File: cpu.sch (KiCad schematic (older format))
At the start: 6 parts

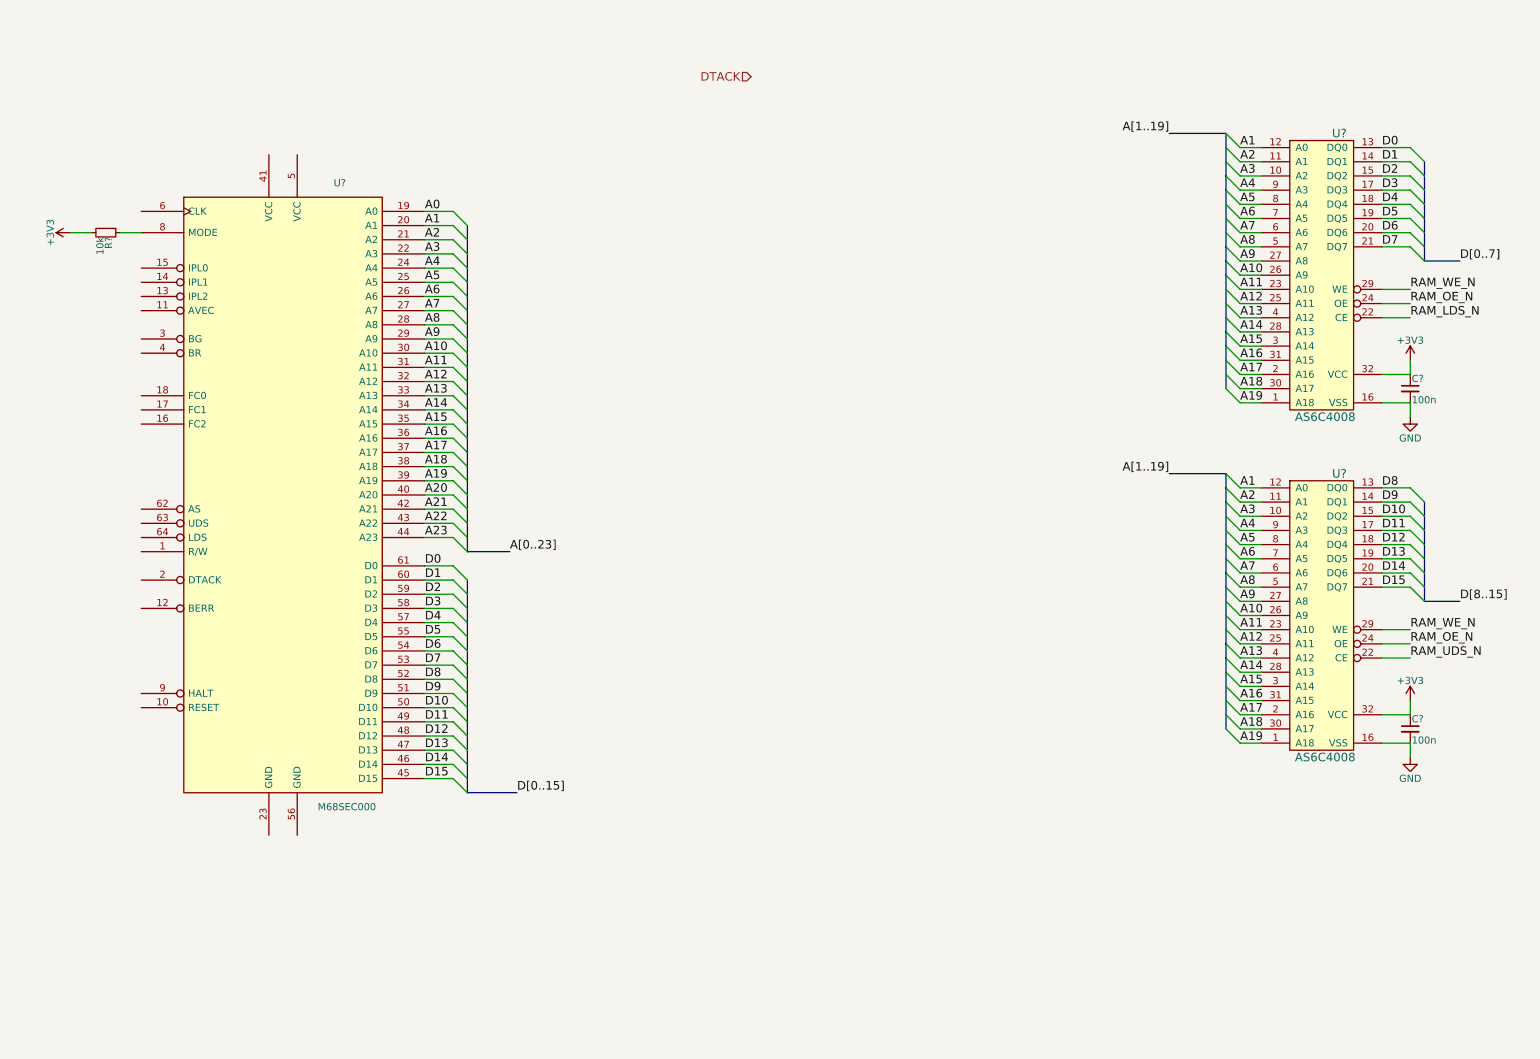
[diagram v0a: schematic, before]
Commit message: boot process
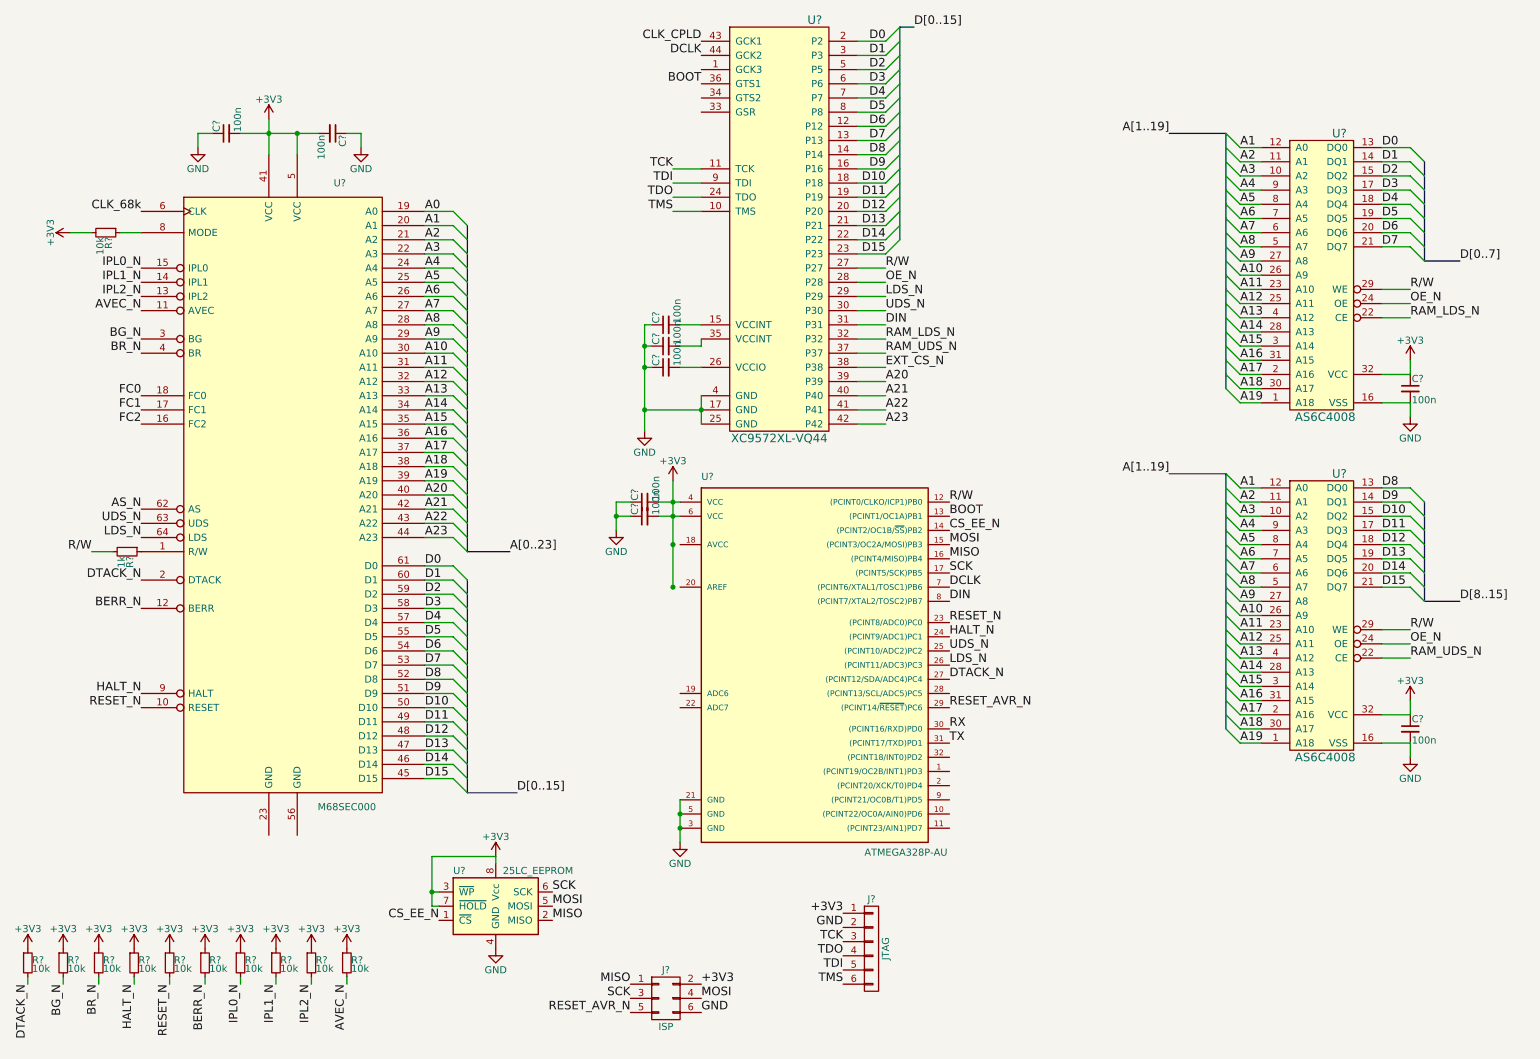
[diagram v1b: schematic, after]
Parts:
- added C? (x7): 100n, symbol C_Small
- added J?: JTAG, symbol CONN_01X06
- added J?: ISP, symbol CONN_02X03
- added R?: 1k, symbol R_Small
- added R? (x10): 10k, symbol R_Small
- added U?: XC9572XL-VQ44, symbol XC9572XL-VQ44
- added U?: ATMEGA328P-AU, TQFP32, symbol ATMEGA328P-AU
- added U?: 25LC_EEPROM, symbol 25LC_EEPROM
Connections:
- net +3V3: now also U?.41 (VCC), U?.5 (VCC), C?.2, C?.2, C?.2, C?.2, J?.1 (P1), J?.2 (P2), R?.1, R?.1, R?.1, R?.1, R?.1, R?.1, R?.1, R?.1, R?.1, R?.1, U?.3 (~WP), U?.4 (VCC), U?.6 (VCC), U?.7 (~HOLD), U?.8 (Vcc)
- net A20: now also U?.39 (P39)
- net A21: now also U?.40 (P40)
- net A22: now also U?.41 (P41)
- net A23: now also U?.42 (P42)
- net D0: now also U?.2 (P2)
- net D1: now also U?.3 (P3)
- net D10: now also U?.18 (P18)
- net D11: now also U?.19 (P19)
- net D12: now also U?.20 (P20)
- net D13: now also U?.21 (P21)
- net D14: now also U?.22 (P22)
- net D15: now also U?.23 (P23)
- net D2: now also U?.5 (P5)
- net D3: now also U?.6 (P6)
- net D4: now also U?.7 (P7)
- net D5: now also U?.8 (P8)
- net D6: now also U?.12 (P12)
- net D7: now also U?.13 (P13)
- net D8: now also U?.14 (P14)
- net D9: now also U?.16 (P16)
- net GND: now also C?.1, C?.1, C?.1, C?.1, C?.1, C?.1, C?.1, J?.2 (P2), J?.6 (P6), U?.17 (GND), U?.21 (GND), U?.25 (GND), U?.3 (GND), U?.4 (GND), U?.4 (GND), U?.5 (GND)
- net RAM_LDS_N: now also U?.32 (P32)
- net RAM_UDS_N: now also U?.37 (P37)
- net at U?.1 (R/W): now also R?.1
- net RESET_N: now reaches U?.10 (RESET)
- net RESET_N: now also R?.2, U?.23 ((PCINT8/ADC0)PC0)
- net AVEC_N: now reaches U?.11 (AVEC)
- net AVEC_N: now also R?.2
- net BERR_N: now reaches U?.12 (BERR)
- net BERR_N: now also R?.2
- net IPL2_N: now reaches U?.13 (IPL2)
- net IPL2_N: now also R?.2
- net IPL1_N: now reaches U?.14 (IPL1)
- net IPL1_N: now also R?.2
- net IPL0_N: now reaches U?.15 (IPL0)
- net IPL0_N: now also R?.2
- net FC2: now reaches U?.16 (FC2)
- net FC1: now reaches U?.17 (FC1)
- net FC0: now reaches U?.18 (FC0)
- net DTACK_N: now reaches U?.2 (DTACK)
- net DTACK_N: now also R?.2, U?.27 ((PCINT12/SDA/ADC4)PC4)
- net BG_N: now reaches U?.3 (BG)
- net BG_N: now also R?.2
- net BR_N: now reaches U?.4 (BR)
- net BR_N: now also R?.2
- net CLK_68k: now reaches U?.6 (CLK)
- net AS_N: now reaches U?.62 (AS)
- net UDS_N: now reaches U?.63 (UDS)
- net UDS_N: now also U?.25 ((PCINT10/ADC2)PC2), U?.30 (P30)
- net LDS_N: now reaches U?.64 (LDS)
- net LDS_N: now also U?.26 ((PCINT11/ADC3)PC3), U?.29 (P29)
- net HALT_N: now reaches U?.9 (HALT)
- net HALT_N: now also R?.2, U?.24 ((PCINT9/ADC1)PC1)
- net RAM_OE_N renamed OE_N
- net OE_N: now also U?.28 (P28)
- net RAM_WE_N renamed R/W
- net R/W: now also R?.2, U?.12 ((PCINT0/CLKO/ICP1)PB0), U?.27 (P27)
- new net: C?.2, U?.15 (VCCINT)
- new net: C?.2, U?.26 (VCCIO)
- new net: C?.2, U?.35 (VCCINT)
- new net BOOT: U?.13 ((PCINT1/OC1A)PB1), U?.36 (GTS1)
- new net CLK_CPLD: U?.43 (GCK1)
- new net CS_EE_N: U?.1 (~CS), U?.14 ((PCINT2/OC1B/~SS~)PB2)
- new net DCLK: U?.44 (GCK2), U?.7 ((PCINT6/XTAL1/TOSC1)PB6)
- new net DIN: U?.31 (P31), U?.8 ((PCINT7/XTAL2/TOSC2)PB7)
- new net EXT_CS_N: U?.38 (P38)
- new net MISO: J?.1 (P1), U?.16 ((PCINT4/MISO)PB4), U?.2 (MISO)
- new net MOSI: J?.4 (P4), U?.15 ((PCINT3/OC2A/MOSI)PB3), U?.5 (MOSI)
- new net RESET_AVR_N: J?.5 (P5), U?.29 ((PCINT14/~RESET~)PC6)
- new net RX: U?.30 ((PCINT16/RXD)PD0)
- new net SCK: J?.3 (P3), U?.17 ((PCINT5/SCK)PB5), U?.6 (SCK)
- new net TCK: J?.3 (P3), U?.11 (TCK)
- new net TDI: J?.5 (P5), U?.9 (TDI)
- new net TDO: J?.4 (P4), U?.24 (TDO)
- new net TMS: J?.6 (P6), U?.10 (TMS)
- new net TX: U?.31 ((PCINT17/TXD)PD1)
